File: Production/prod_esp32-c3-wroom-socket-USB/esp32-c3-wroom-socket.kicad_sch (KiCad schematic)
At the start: 22 parts, among them J1 USB-C_Receptacle_Data_16P_GCT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, J3 USB-C_KUSBX-SL-CS1N14-B, J4 USB-C_Receptacle_Data_16P_GCT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, SW1 SW_Push_SMD_6x3.5, SW2 SW_Push_SMD_6x3.5, U1 ESP32-C3-WROOM-02-N4, U2 AMS1117-3V3

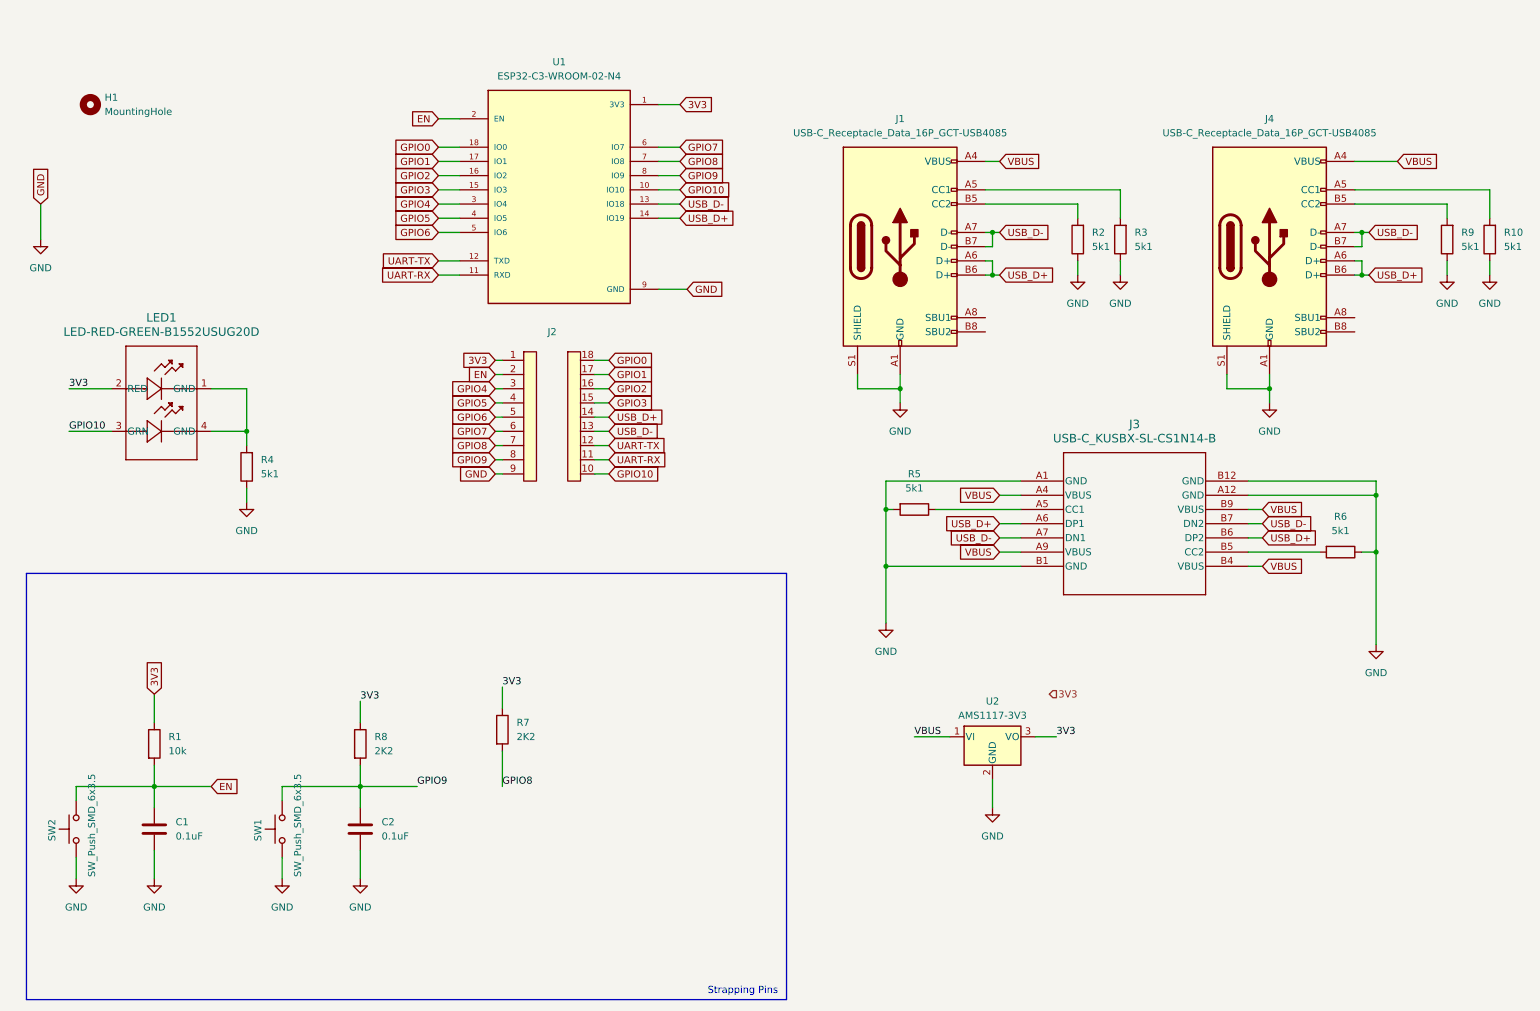
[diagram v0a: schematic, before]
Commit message: esp32-c3 zen
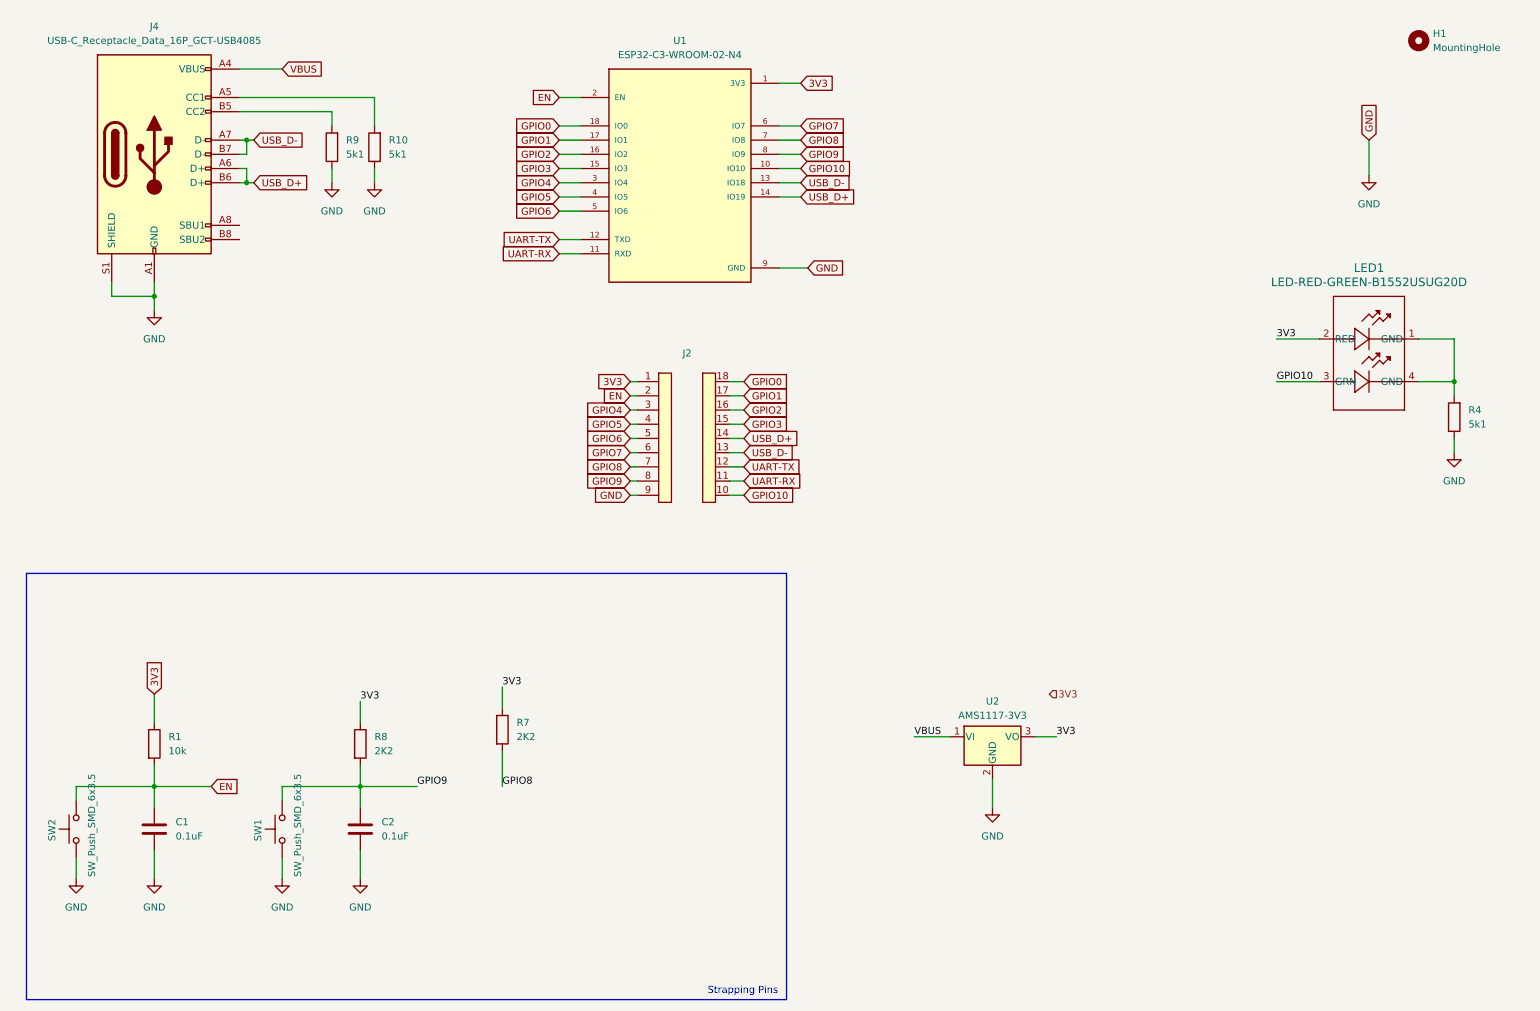
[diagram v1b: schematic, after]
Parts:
- removed J1: USB-C_Receptacle_Data_16P_GCT-USB4085, Alexander Footprint Library:USB-C GCT CONN16_USB4085-GF-A, symbol Alexander Symbol Library:USB-C_Receptacle_Data_16P_GCT-USB4085
- removed J3: USB-C_KUSBX-SL-CS1N14-B, Alexander Footprint Library:USB-C_KUSBX-SL-CS1N14-B_KYC, symbol Alexander_Library_Symbols:USB-C_KUSBX-SL-CS1N14-B
- removed R2, R3, R5, R6: 5k1, Resistor_SMD:R_1206_3216Metric_Pad1.30x1.75mm_HandSolder, symbol Device:R
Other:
- moved on the sheet: H1, J2, J4, LED1, R10, R4, R9, U1

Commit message: esp32-c3 zen
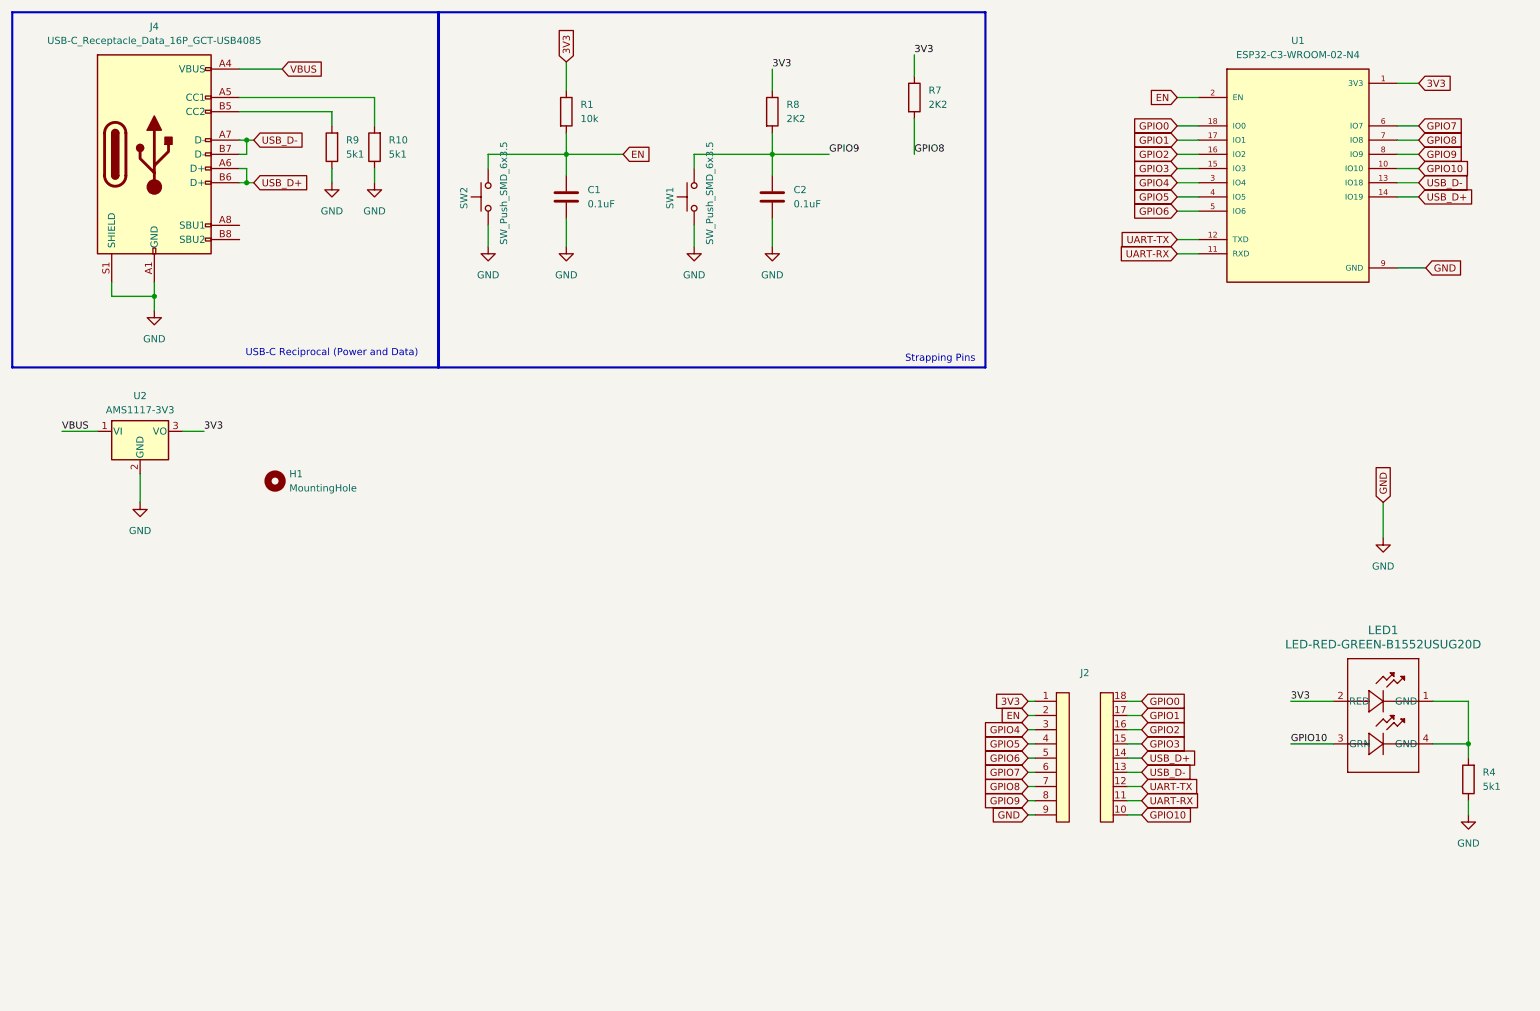
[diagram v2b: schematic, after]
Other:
- note added: "USB-C Reciprocal (Power and Data)"
- moved on the sheet: C1, C2, H1, J2, LED1, R1, R4, R7, R8, SW1, SW2, U1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
